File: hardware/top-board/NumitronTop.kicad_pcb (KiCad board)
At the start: 2 copper layers, 110 x 30 mm, 4 parts

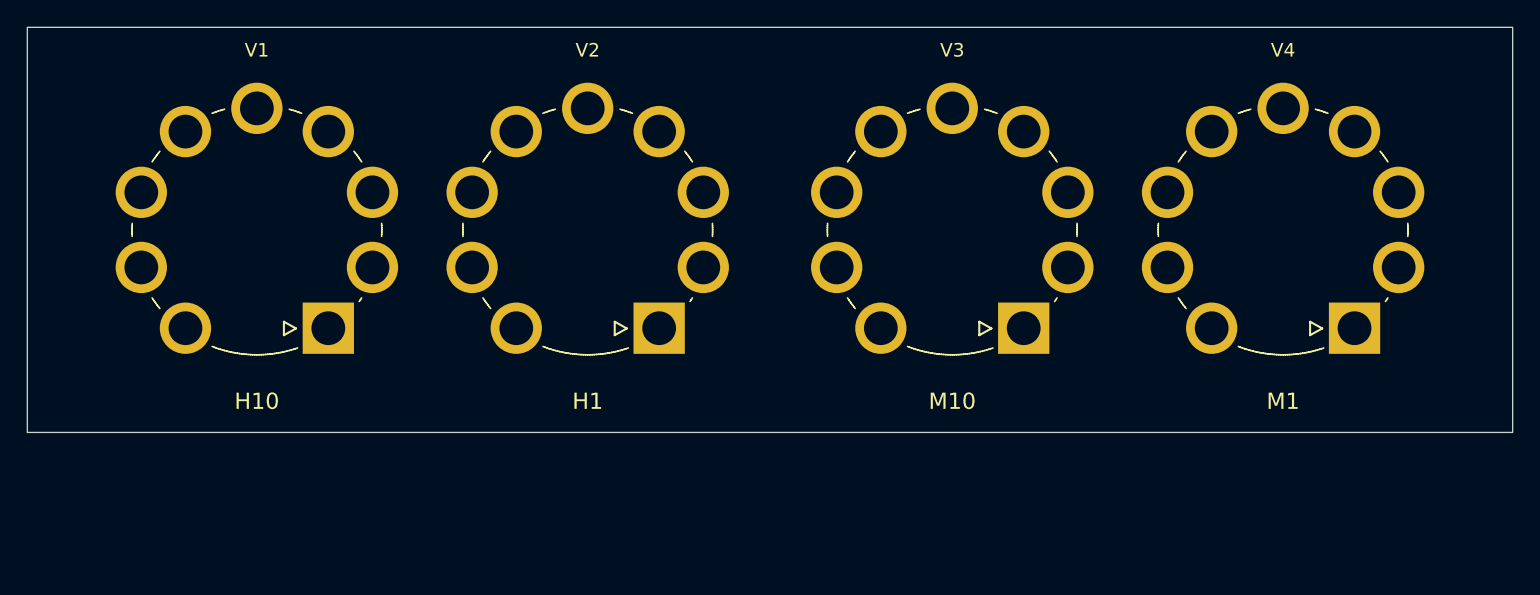
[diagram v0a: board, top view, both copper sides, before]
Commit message: Complete routed top-board prototype layout
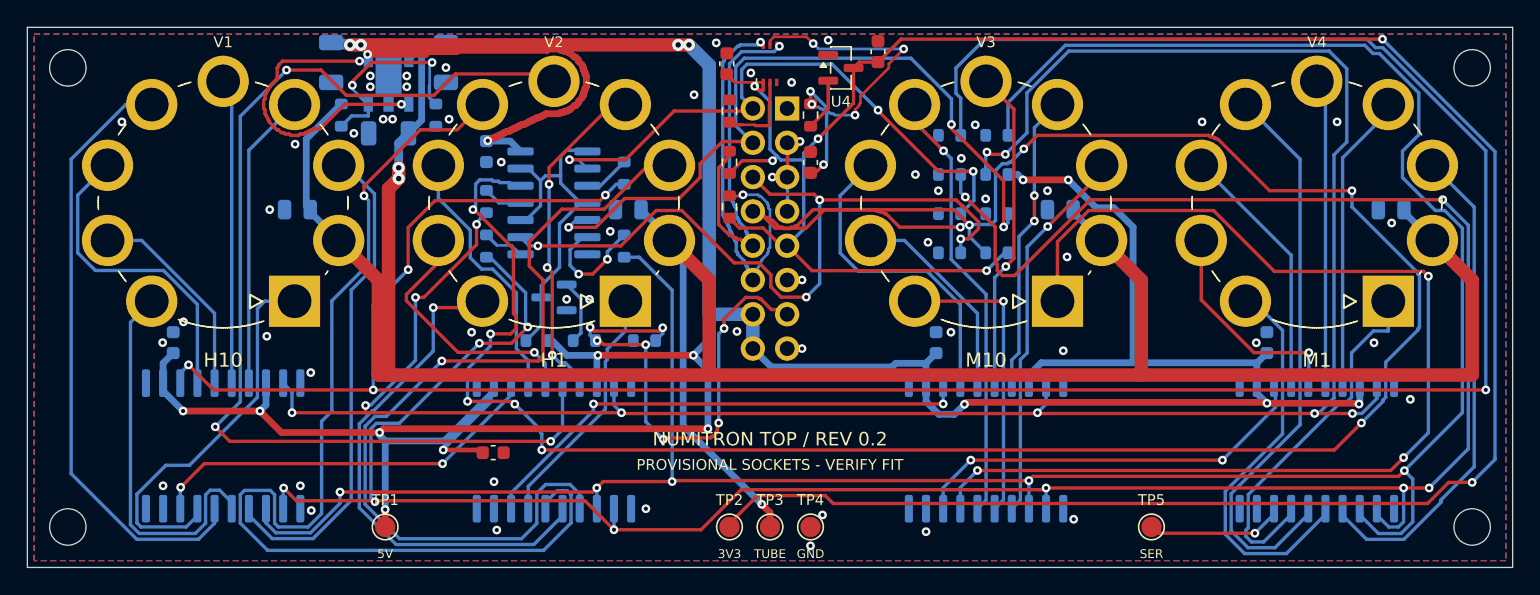
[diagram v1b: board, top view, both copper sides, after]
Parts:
- added C1: 10u 25V X7R, Capacitor_SMD:C_1206_3216Metric, B.Cu at (72.5, 52.6)
- added C10: 100n 50V X7R, Capacitor_SMD:C_0603_1608Metric, F.Cu at (84.5, 81.5)
- added C11: 1u 25V X7R, Capacitor_SMD:C_0805_2012Metric, B.Cu at (94.5, 63.5)
- added C12: 100n 50V X7R, Capacitor_SMD:C_0603_1608Metric, B.Cu at (117.3, 73.3)
- added C13: 1u 25V X7R, Capacitor_SMD:C_0805_2012Metric, B.Cu at (126.5, 63.5)
- added C14: 100n 50V X7R, Capacitor_SMD:C_0603_1608Metric, B.Cu at (141.8, 73.3)
- added C15: 1u 25V X7R, Capacitor_SMD:C_0805_2012Metric, B.Cu at (151.0, 63.5)
- added C2: 10u 25V X7R, Capacitor_SMD:C_1206_3216Metric, B.Cu at (81.0, 52.6)
- added C3: 10u 25V X7R, Capacitor_SMD:C_1206_3216Metric, B.Cu at (76.8, 57.9)
- added C4: 100n 50V X7R, Capacitor_SMD:C_0603_1608Metric, B.Cu at (84.0, 59.2)
- added C5: 100n 50V X7R, Capacitor_SMD:C_0603_1608Metric, F.Cu at (101.8, 52.7)
- added C6: 100n 50V X7R, Capacitor_SMD:C_0603_1608Metric, F.Cu at (108.0, 60.0)
- added C7: 100n 50V X7R, Capacitor_SMD:C_0603_1608Metric, F.Cu at (113.0, 51.8)
- added C8: 100n 50V X7R, Capacitor_SMD:C_0603_1608Metric, B.Cu at (60.8, 73.3)
- added C9: 1u 25V X7R, Capacitor_SMD:C_0805_2012Metric, B.Cu at (70.0, 63.5)
- added H1: M2.5 / NPTH 2.7, Numitron:MountingHole_2.7mm_M2.5_BothSides, F.Cu at (53.0, 53.0)
- added H2: M2.5 / NPTH 2.7, Numitron:MountingHole_2.7mm_M2.5_BothSides, F.Cu at (157.0, 53.0)
- added H3: M2.5 / NPTH 2.7, Numitron:MountingHole_2.7mm_M2.5_BothSides, F.Cu at (53.0, 87.0)
- added H4: M2.5 / NPTH 2.7, Numitron:MountingHole_2.7mm_M2.5_BothSides, F.Cu at (157.0, 87.0)
- added J1: 61201621621, Numitron:Wurth_61201621621_2x08_P2.54mm, B.Cu at (106.3, 56.0)
- added Q1: MMBT3904-7-F, Package_TO_SOT_SMD:SOT-23, B.Cu at (89.0, 70.0)
- added R1: 46.4k 1%, Resistor_SMD:R_0603_1608Metric, B.Cu at (73.2, 56.5)
- added R10: 2.2k, Resistor_SMD:R_0603_1608Metric, B.Cu at (121.8, 60.9)
- added R11: 4.7k, Resistor_SMD:R_0603_1608Metric, B.Cu at (118.3, 63.8)
- added R12: 4.7k, Resistor_SMD:R_0603_1608Metric, B.Cu at (121.8, 63.8)
- added R13: 4.7k, Resistor_SMD:R_0603_1608Metric, B.Cu at (118.3, 66.7)
- added R14: 4.7k, Resistor_SMD:R_0603_1608Metric, B.Cu at (121.8, 66.7)
- added R15: 1k, Resistor_SMD:R_0603_1608Metric, B.Cu at (87.8, 73.2)
- added R16: 2.2k, Resistor_SMD:R_0603_1608Metric, B.Cu at (91.2, 73.2)
- added R17: 4.7k, Resistor_SMD:R_0603_1608Metric, B.Cu at (95.7, 73.2)
- added R18: 1k, Resistor_SMD:R_0603_1608Metric, F.Cu at (108.0, 56.5)
- added R19: 10k, Resistor_SMD:R_0603_1608Metric, F.Cu at (102.0, 56.2)
- added R2: 10k 1%, Resistor_SMD:R_0603_1608Metric, B.Cu at (80.2, 56.5)
- added R20: 4.7k, Resistor_SMD:R_0603_1608Metric, F.Cu at (102.0, 60.0)
- added R21: 4.7k, Resistor_SMD:R_0603_1608Metric, F.Cu at (102.0, 63.3)
- added R3: 33R, Resistor_SMD:R_0603_1608Metric, B.Cu at (94.2, 60.8)
- added R4: 33R, Resistor_SMD:R_0603_1608Metric, B.Cu at (94.2, 66.2)
- added R5: 33R, Resistor_SMD:R_0603_1608Metric, B.Cu at (84.0, 66.2)
- added R6: 33R, Resistor_SMD:R_0603_1608Metric, B.Cu at (84.0, 62.9)
- added R7: 100k, Resistor_SMD:R_0603_1608Metric, B.Cu at (118.3, 58.0)
- added R8: 100k, Resistor_SMD:R_0603_1608Metric, B.Cu at (121.8, 58.0)
- added R9: 100k, Resistor_SMD:R_0603_1608Metric, B.Cu at (118.3, 60.9)
- added TP1: +5V, TestPoint:TestPoint_Pad_D1.5mm, F.Cu at (76.5, 87.0)
- added TP2: +3V3, TestPoint:TestPoint_Pad_D1.5mm, F.Cu at (102.0, 87.0)
- added TP3: V_TUBE, TestPoint:TestPoint_Pad_D1.5mm, F.Cu at (105.0, 87.0)
- added TP4: GND, TestPoint:TestPoint_Pad_D1.5mm, F.Cu at (108.0, 87.0)
- added TP5: SER_OUT 5V, TestPoint:TestPoint_Pad_D1.5mm, F.Cu at (133.2, 87.0)
- added U1: AP7361C-Y5-13, Numitron:Diodes_SOT89-5_AP7361C, B.Cu at (76.8, 54.0)
- added U2: SN74AHCT125DR, Package_SO:SOIC-14_3.9x8.7mm_P1.27mm, B.Cu at (89.0, 63.0)
- added U3: BH1750FVI-TR, Numitron:ROHM_WSOF6I_BH1750_NoCenterPad, F.Cu at (105.0, 52.7)
- added U4: TLV809EA29DBZR, Package_TO_SOT_SMD:SOT-23, F.Cu at (110.2, 53.0)
- added U5: TPIC6B595DWR, Package_SO:SOIC-20W_7.5x12.8mm_P1.27mm, B.Cu at (64.5, 81.0)
- added U6: TPIC6B595DWR, Package_SO:SOIC-20W_7.5x12.8mm_P1.27mm, B.Cu at (89.0, 81.0)
- added U7: TPIC6B595DWR, Package_SO:SOIC-20W_7.5x12.8mm_P1.27mm, B.Cu at (121.0, 81.0)
- added U8: TPIC6B595DWR, Package_SO:SOIC-20W_7.5x12.8mm_P1.27mm, B.Cu at (145.5, 81.0)
- moved V1 3.20 mm to (64.5, 63.0)
- moved V2 3.20 mm to (89.0, 63.0)
- moved V3 3.20 mm to (121.0, 63.0)
- moved V4 3.20 mm to (145.5, 63.0)
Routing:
- net +5V: track 0.00 -> 302.0 mm, vias 0 -> 21
- net V_TUBE: track 0.00 -> 201.2 mm, vias 0 -> 3
- net SER_5V: track 0.00 -> 195.3 mm, vias 0 -> 5
- net RCK_5V: track 0.00 -> 191.5 mm, vias 0 -> 10
- net SRCK_5V: track 0.00 -> 188.3 mm, vias 0 -> 5
- net +3V3: track 0.00 -> 188.3 mm, vias 0 -> 6
- net BLANK_3V3: track 0.00 -> 186.8 mm, vias 0 -> 10
- net BLANK_5V: track 0.00 -> 169.0 mm, vias 0 -> 10
- net /Four tube drivers/M10_DP: track 0.00 -> 84.4 mm, vias 0 -> 3
- net /Four tube drivers/H1_C: track 0.00 -> 80.0 mm, vias 0 -> 3
- net /Four tube drivers/H1_G: track 0.00 -> 79.3 mm, vias 0 -> 1
- net /Four tube drivers/H1_E: track 0.00 -> 64.0 mm, vias 0 -> 1
- net RCK_3V3: track 0.00 -> 54.6 mm, vias 0 -> 4
- net SRCK_3V3: track 0.00 -> 54.4 mm, vias 0 -> 3
- net /Four tube drivers/H10_G: track 0.00 -> 45.1 mm
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- added copper zone on B.Cu, net GND
- added copper zone on F.Cu, net GND
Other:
- board size 110 x 30 mm -> 110 x 40 mm
- board text added: "3V3"
- board text added: "5V"
- board text added: "GND"
- board text added: "J1 REV 0.1"
- board text added: "NUMITRON TOP / REV 0.2"
- board text added: "PROVISIONAL SOCKETS - VERIFY FIT"
- board text added: "SER"
- board text added: "TUBE"
